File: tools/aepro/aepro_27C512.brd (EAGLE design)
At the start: 53 x 76.2 mm, 22 parts, among them IC1 MCP23017SP, IC2 MCP23008/P, U1 328P, Y1 16 MHz

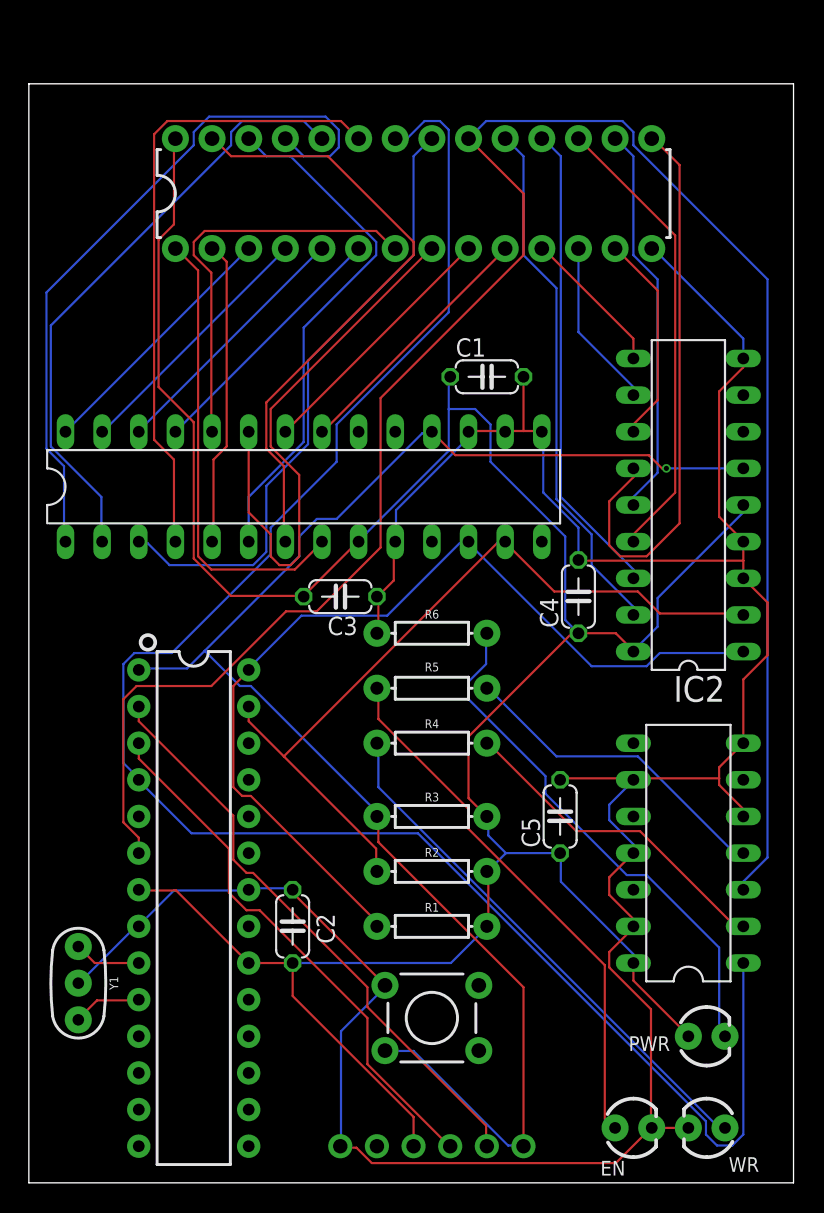
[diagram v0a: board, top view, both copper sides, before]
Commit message: AEPRO rev 7
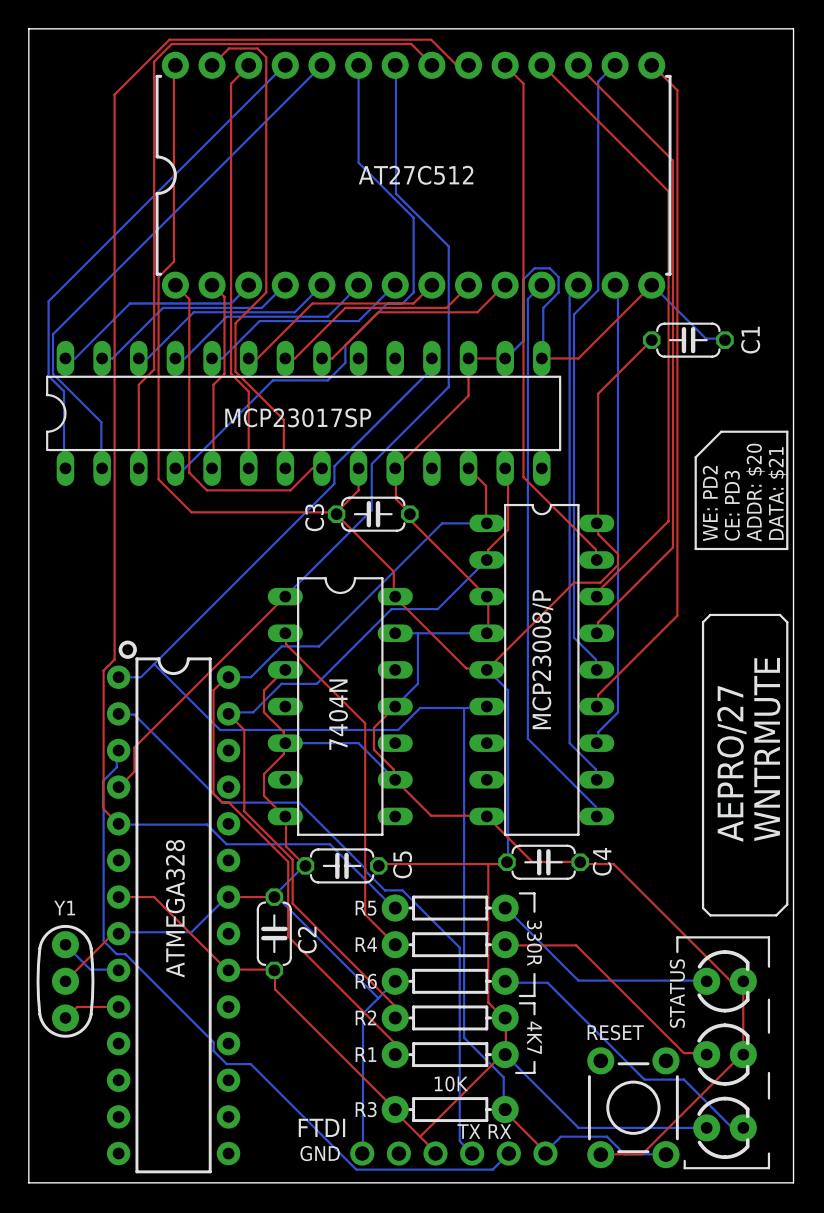
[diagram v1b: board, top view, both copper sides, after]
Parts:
- U$1: device wntrmute:DIL28-3-ZIF_SOCKET -> wntrmute:DIL28-6-ZIF_SOCKET
- moved V1 26.2 mm to (21.6, 33.0), turned to 270 degrees
- moved R6 24.2 mm to (29.2, 14.0)
- moved R3 20.4 mm to (29.2, 5.08), turned to 0 degrees
- moved C4 18.6 mm to (35.7, 22.2), turned to 0 degrees
- moved C5 15.5 mm to (21.7, 22.0), turned to 180 degrees
- moved S1 15.3 mm to (41.9, 5.21), turned to 90 degrees
- moved IC2 15.3 mm to (35.6, 35.6), turned to 270 degrees
- moved R5 15.3 mm to (29.2, 19.1), turned to 0 degrees
- moved C1 14.2 mm to (45.7, 58.4)
- moved R4 14.0 mm to (29.2, 16.5), turned to 0 degrees
- moved D4 12.0 mm to (48.3, 14.0), flipped to the bottom, turned to 180 degrees
- moved R2 10.2 mm to (29.2, 11.4)
- moved R1 8.98 mm to (29.2, 8.89)
- moved D1 6.48 mm to (48.3, 3.81)
- moved C3 6.16 mm to (23.9, 46.4)
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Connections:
- removed net N$12: CN1.5, U1.2
- removed net N$3: R5.P$1, V1.4
- new net N$11: CN1.5, U1.3
- net GND: now also V1.3
- net N$4: now also R5.P$1, U1.5; no longer U1.6, V1.3
- net N$6: now also U1.2; no longer U1.3
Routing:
- net N$2: track 126.0 -> 61.1 mm
- net N$11: track 0.00 -> 49.1 mm
- net N$12: track 40.7 -> 0.00 mm
- net N$4: track 136.6 -> 99.8 mm
- net D0: track 10.3 -> 39.2 mm
- net A2: track 38.6 -> 14.8 mm
- net D1: track 11.7 -> 35.3 mm
- net N$3: track 22.5 -> 0.00 mm
- net N$9: track 37.4 -> 16.1 mm
- net N$1: track 37.0 -> 17.1 mm
- net D2: track 14.6 -> 32.5 mm
- net D4: track 27.3 -> 43.8 mm
- net N$10: track 36.7 -> 20.7 mm
- net A8: track 49.8 -> 35.3 mm
- net A3: track 28.5 -> 14.8 mm
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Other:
- board size 53 x 76.2 mm -> 53 x 80 mm
- board text added: "10K"
- board text added: "330R"
- board text added: "4K7"
- board text added: "AEPRO/27"
- board text added: "AT27C512"
- board text added: "ATMEGA328"
- board text added: "FTDI"
- board text added: "GND"
- board text added: "K_ISOM/OAK_CA"
- board text added: "RESET"
- board text added: "REV7/20191002"
- board text added: "RX"
- board text added: "STATUS"
- board text added: "TX"
- board text added: "WE: PD2 CE: PD3 ADDR: $20 DATA: $21"
- board text added: "WNTRMUTE"
- board text added: "Y1"
- board text removed: "EN"
- board text removed: "PWR"
- board text removed: "WR"
